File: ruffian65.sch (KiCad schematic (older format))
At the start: 21 parts, among them J1 AVR-ISP-6, SW70 SW_Push, U1 ATmega32U4-MU, Y1 Crystal_GND24_Small

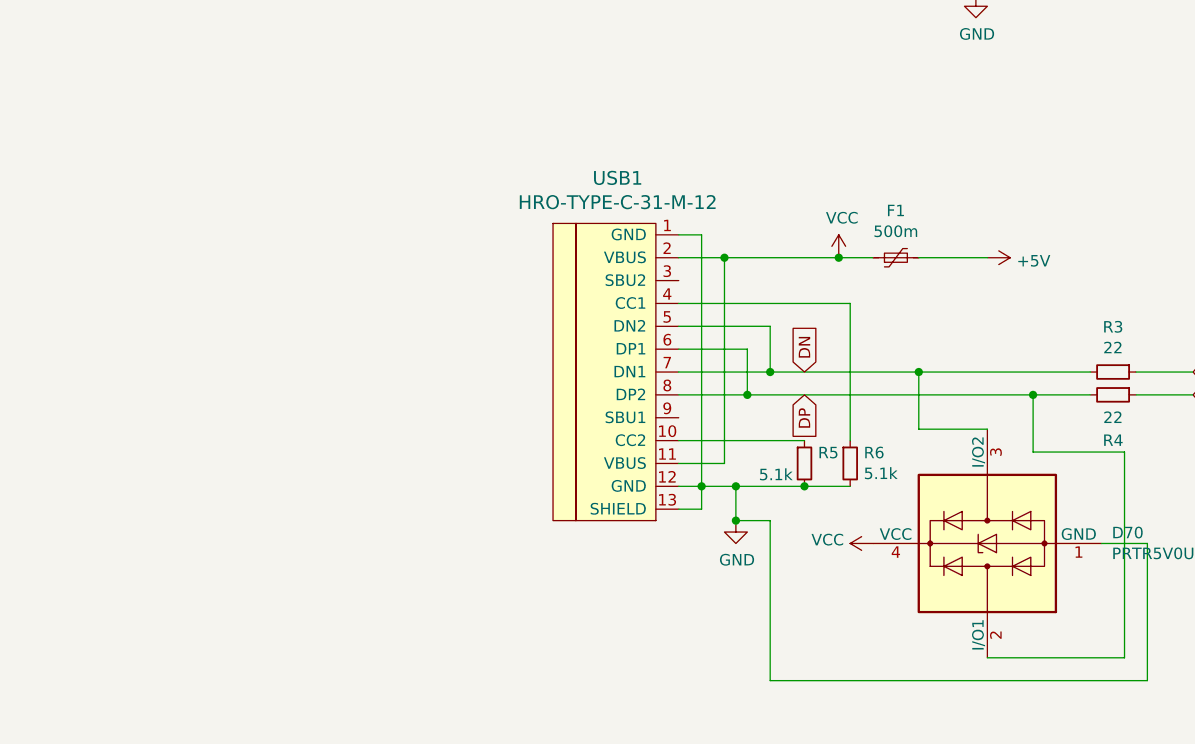
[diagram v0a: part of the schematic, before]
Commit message: encoder support?
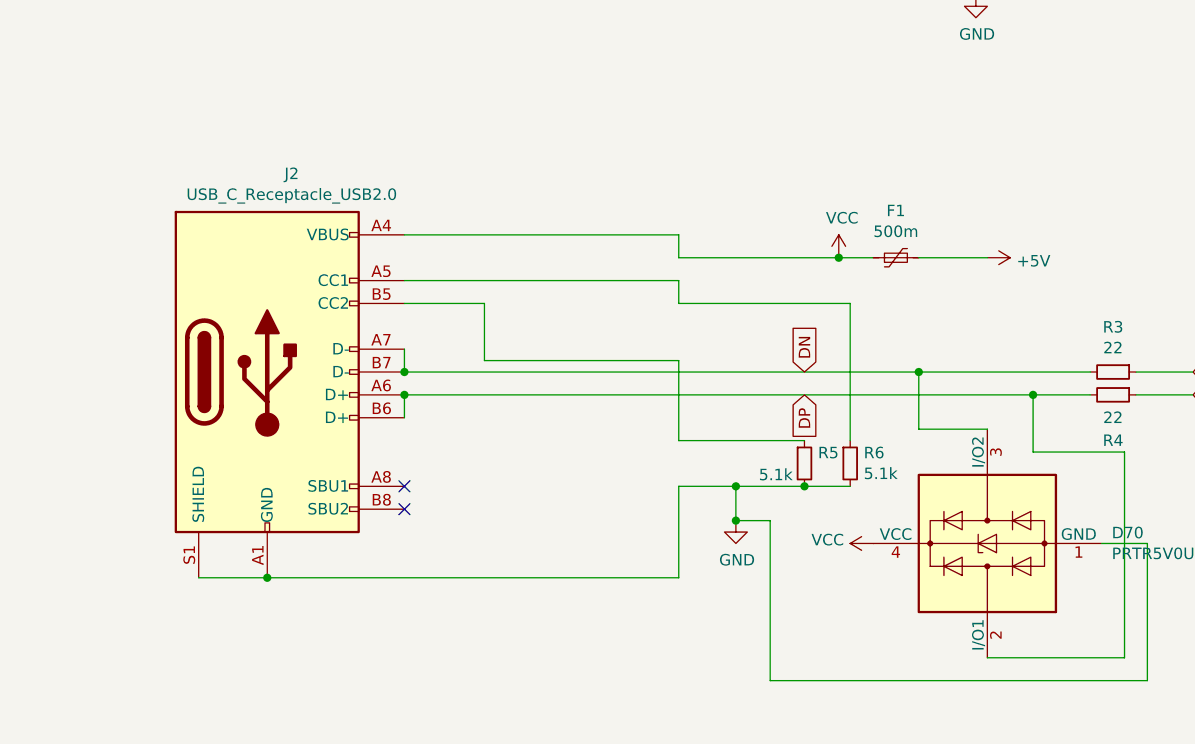
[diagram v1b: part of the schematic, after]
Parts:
- removed USB1: HRO-TYPE-C-31-M-12, Type-C:HRO-TYPE-C-31-M-12-HandSoldering, symbol Type-C:HRO-TYPE-C-31-M-12
- added J2: USB_C_Receptacle_USB2.0, Connector_USB:USB_C_Receptacle_HRO_TYPE-C-31-M-12, symbol Connector:USB_C_Receptacle_USB2.0
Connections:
- net DN: now also J2.A7 (D-), J2.B7 (D-)
- net DP: now also J2.A6 (D+), J2.B6 (D+)
- net GND: now also J2.A1 (GND), J2.A12 (GND), J2.B1 (GND), J2.B12 (GND), J2.S1 (SHIELD)
- net VCC: now also J2.A4 (VBUS), J2.A9 (VBUS), J2.B4 (VBUS), J2.B9 (VBUS)
- net at R5.1: now also J2.B5 (CC2)
- net at R6.1: now also J2.A5 (CC1)
- no-connect marks 0 -> 2
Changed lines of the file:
@@
 	7200 1500 7200 1650
-$Comp
-L Type-C:HRO-TYPE-C-31-M-12 USB1
-U 1 1 6139D968
-P 5800 3250
-F 0 "USB1" H 5633 4047 60  0000 C CNN
-F 1 "HRO-TYPE-C-31-M-12" H 5633 3941 60  0000 C CNN
-F 2 "Type-C:HRO-TYPE-C-31-M-12-HandSoldering" H 5800 3250 60  0001 C CNN
-F 3 "" H 5800 3250 60  0001 C CNN
-	1    5800 3250
-	1    0    0    -1
-$EndComp
 $Comp
 L Device:R_Small R3
@@
 Wire Wire Line
 	7900 3400 8150 3400
-Wire Wire Line
-	5900 2700 6000 2700
-Wire Wire Line
-	6000 2700 6000 3800
-Wire Wire Line
-	6000 3800 5900 3800
-Wire Wire Line
-	5900 3900 6000 3900
-Wire Wire Line
-	6000 3900 6000 3800
-Connection ~ 6000 3800
 $Comp
 L power:VCC #PWR0112
@@
 	1    0    0    -1
 $EndComp
-Wire Wire Line
-	5900 2800 6100 2800
-Wire Wire Line
-	5900 3400 6200 3400
-Wire Wire Line
-	5900 3300 6300 3300
-Wire Wire Line
-	5900 3100 6300 3100
-Wire Wire Line
-	6300 3100 6300 3300
-Wire Wire Line
-	5900 3200 6200 3200
-Wire Wire Line
-	6200 3200 6200 3400
-Wire Wire Line
-	5900 3700 6100 3700
-Wire Wire Line
-	6100 3700 6100 2800
-Connection ~ 6100 2800
-Wire Wire Line
-	6100 2800 6600 2800
 $Comp
 L Device:Polyfuse_Small F1
@@
 $EndComp
 Wire Wire Line
-	5900 3600 6450 3600
-Wire Wire Line
-	6000 3800 6150 3800
-Wire Wire Line
 	6450 3800 6650 3800
 Connection ~ 6450 3800
@@
 Wire Wire Line
 	6150 3800 6450 3800
-Wire Wire Line
-	6300 3300 6950 3300
-Connection ~ 6300 3300
-Wire Wire Line
-	6200 3400 7450 3400
-Connection ~ 6200 3400
 $Comp
 L Power_Protection:PRTR5V0U2X D70
@@
 Text GLabel 10250 1900 2    50   Input ~ 0
 rot1
+$Comp
+L Connector:USB_C_Receptacle_USB2.0 J2
+U 1 1 613F3603
+P 4100 3300
+F 0 "J2" H 4207 4167 50  0000 C CNN
+F 1 "USB_C_Receptacle_USB2.0" H 4207 4076 50  0000 C CNN
+F 2 "Connector_USB:USB_C_Receptacle_HRO_TYPE-C-31-M-12" H 4250 3300 50  0001 C CNN
+F 3 "https://www.usb.org/sites/default/files/documents/usb_type-c.zip" H 4250 3300 50  0001 C CNN
+	1    4100 3300
+	1    0    0    -1
+$EndComp
+Wire Wire Line
+	5900 3600 6450 3600
+NoConn ~ 4700 3900
+NoConn ~ 4700 3800
+Wire Wire Line
+	4700 3500 4700 3400
+Connection ~ 4700 3400
+Wire Wire Line
+	4700 3300 4700 3200
+Connection ~ 4700 3300
+Wire Wire Line
+	4700 3400 7450 3400
+Wire Wire Line
+	4700 3300 6950 3300
+Wire Wire Line
+	4100 4200 5900 4200
+Wire Wire Line
+	5900 3800 5900 4200
+Wire Wire Line
+	5900 3800 6150 3800
+Wire Wire Line
+	4700 2700 5900 2700
+Wire Wire Line
+	5900 2700 5900 2800
+Wire Wire Line
+	4700 2900 5900 2900
+Wire Wire Line
+	5900 2900 5900 3000
+Wire Wire Line
+	4700 3000 5050 3000
+Wire Wire Line
+	5050 3000 5050 3250
+Wire Wire Line
+	5050 3250 5900 3250
+Wire Wire Line
+	5900 3250 5900 3600
+Wire Wire Line
+	5900 2800 6600 2800
+Wire Wire Line
+	3800 4200 4100 4200
+Connection ~ 4100 4200
 $EndSCHEMATC
